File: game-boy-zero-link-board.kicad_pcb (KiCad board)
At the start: 2 copper layers, 85.5 x 26 mm, 6 parts, among them J1 GBA_Link, J2 DMG_Link, J3 Breakout, SW1 SW_SPDT, U1 Pico_Reduced, U2 BOB-12009

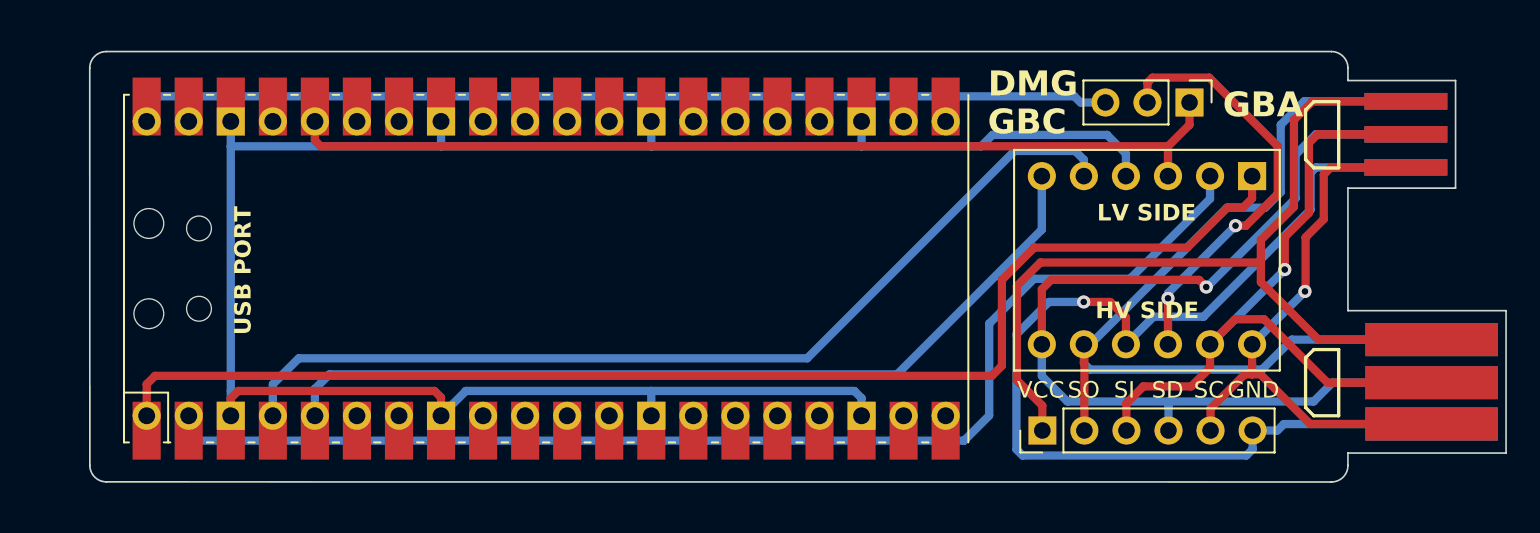
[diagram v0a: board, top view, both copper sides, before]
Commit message: commit local changes (untested)
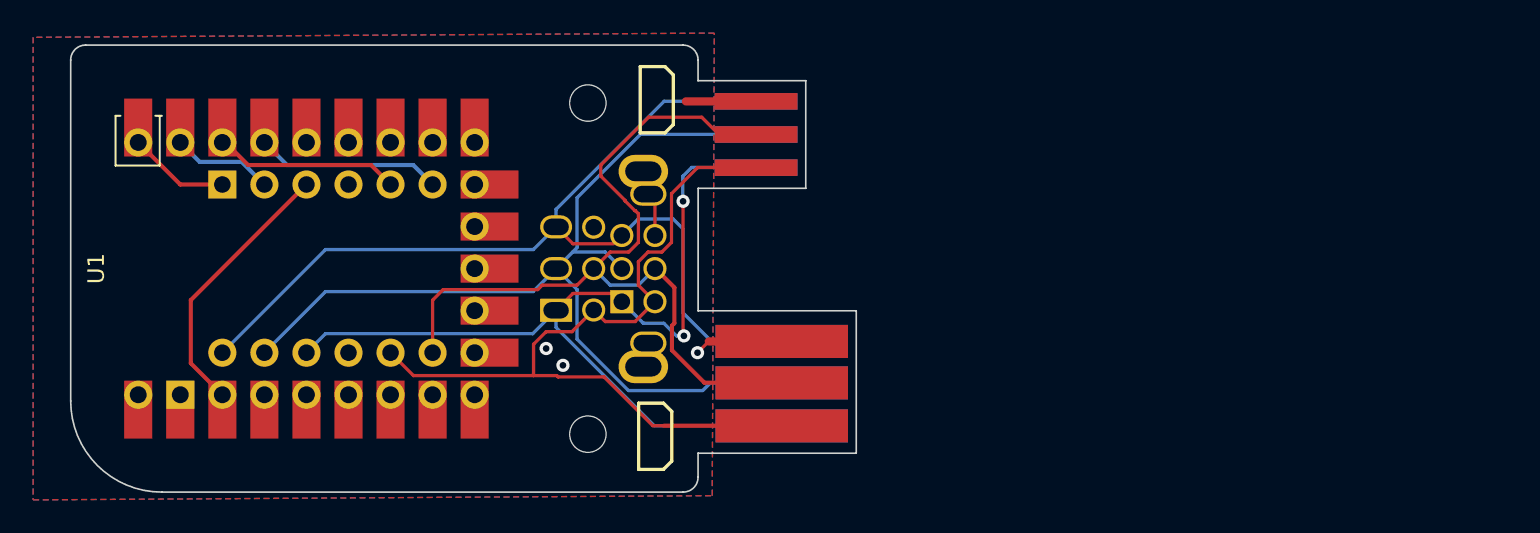
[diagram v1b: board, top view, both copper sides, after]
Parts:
- removed SW1: SW_SPDT, Connector_PinHeader_2.54mm:PinHeader_1x03_P2.54mm_Vertical
- added REF**: MountingHole_2.2mm_M2, MountingHole:MountingHole_2.2mm_M2, F.Cu at (99.5, 85.9)
- added REF**: MountingHole_2.2mm_M2, MountingHole:MountingHole_2.2mm_M2, F.Cu at (99.5, 105.9)
- J1, J2: moved to F.Cu
- J3: value Breakout -> GB_IDC_port; footprint Connector_PinHeader_2.54mm:PinHeader_1x06_P2.54mm_Vertical -> gb-link-socket:GameBoy_LinkPort_DMG_MGB_IDC_Horizontal; moved to B.Cu
- U1: value Pico_Reduced -> RP2040-Zero; footprint MCU_RaspberryPi_and_Boards:RPi_Pico_SMD_TH_REDUCED -> MCU_RaspberryPi_and_Boards:RP2040-Zero_SMD_TH
- Ue: renamed from U2; moved to B.Cu
- moved Ue 49.6 mm to (83.8, 96.3)
- moved J1 39.3 mm to (109.7, 87.8), turned to 90 degrees
- moved J2 39.3 mm to (111.3, 102.8), turned to 90 degrees
- moved J3 26.0 mm to (102.9, 95.9), turned to 0 degrees
- moved U1 14.5 mm to (82.5, 95.9)
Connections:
- J1 pad 6: GND1 -> GND
- J2 pad 6: GND1 -> GND
- J3 pad 6: GND1 -> GND
- U1 pad 13: GND -> unconnected-(U1-GPIO12-Pad13)
- U1 pad 18: GND -> unconnected-(U1-GPIO27_ADC1-Pad18)
- U1 pad 21: unconnected-(U1-GPIO16-Pad21) -> +3.3V
- U1 pad 22: unconnected-(U1-GPIO17-Pad22) -> GND
- U1 pad 23: GND -> unconnected-(U1-VBUS-Pad23)
- U1 pad 3: GND -> /PSO
- U1 pad 4: /PSO -> /PSD
- U1 pad 5: /PSD -> unconnected-(U1-GPIO4-Pad5)
- U1 pad 8: GND -> unconnected-(U1-GPIO7-Pad8)
- Ue pad 10: GND1 -> GND
- Ue pad 9: VCCLOGIC -> /GBVCC
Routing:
- net GND: track 122.4 -> 15.3 mm, vias 0 -> 3
- net /PSC: track 77.7 -> 6.13 mm
- net /PSI: track 73.6 -> 6.13 mm
- net GND1: track 65.7 -> 0.00 mm, vias 1 -> 0
- net +5V: track 59.4 -> 0.00 mm
- net /PSO: track 57.9 -> 11.2 mm
- net /PSD: track 52.8 -> 11.2 mm
- net +3.3V: track 57.8 -> 16.4 mm
- net VCCLOGIC: track 26.0 -> 0.00 mm, vias 2 -> 0
- net /SC: track 35.8 -> 57.6 mm, vias 1 -> 0
- net /SI: track 45.3 -> 57.4 mm, vias 1 -> 0
- net /SD: track 59.4 -> 49.6 mm, vias 1 -> 0
- net /SO: track 56.3 -> 48.8 mm
- net /GBVCC: track 54.3 -> 55.2 mm, vias 0 -> 2
- added copper zone on B.Cu, net GND
- added copper zone on F.Cu, net GND
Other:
- board size 85.5 x 26 mm -> 47.5 x 27 mm
- board text added: "GBZEROLINK AM1 2024"
- board text removed: "DMG"
- board text removed: "GBA"
- board text removed: "GBC"
- board text removed: "GND"
- board text removed: "HV SIDE"
- board text removed: "LV SIDE"
- board text removed: "SC"
- board text removed: "SD"
- board text removed: "SI"
- board text removed: "SO"
- board text removed: "USB PORT"
- board text removed: "USB TO GAMEBOY LINK CABLE ADAPTER"
- board text removed: "VCC"
- board text removed: "agtbaskara.com"
- board text removed: "version 1.6 2023"
